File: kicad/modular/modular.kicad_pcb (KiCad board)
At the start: 2 copper layers, 50.5 x 78 mm, 53 parts, among them J1 CONN_PWR, J2 HEADER, J3 HEADER, U1 LM317, U2 LM337, U3 REF5010, U4 OPA4197

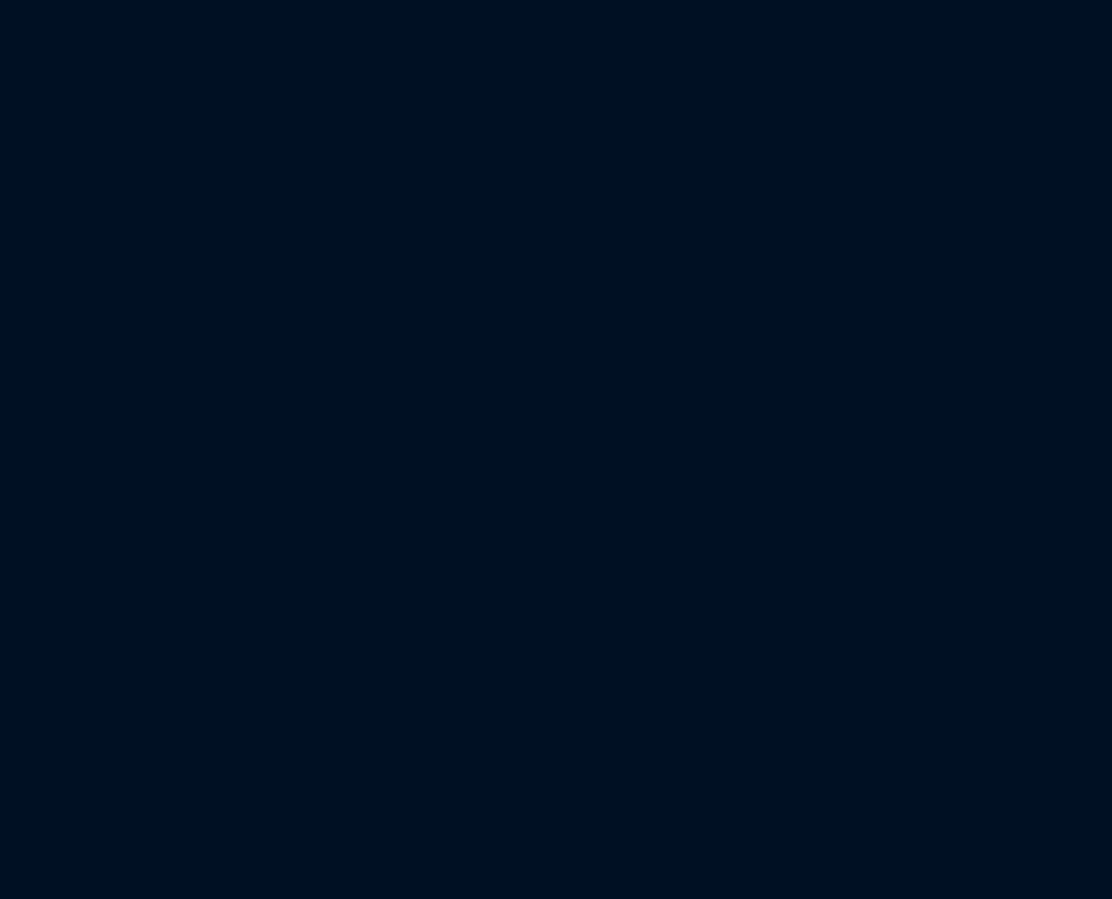
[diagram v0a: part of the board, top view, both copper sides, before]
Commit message: added pcb design of arithmetic board
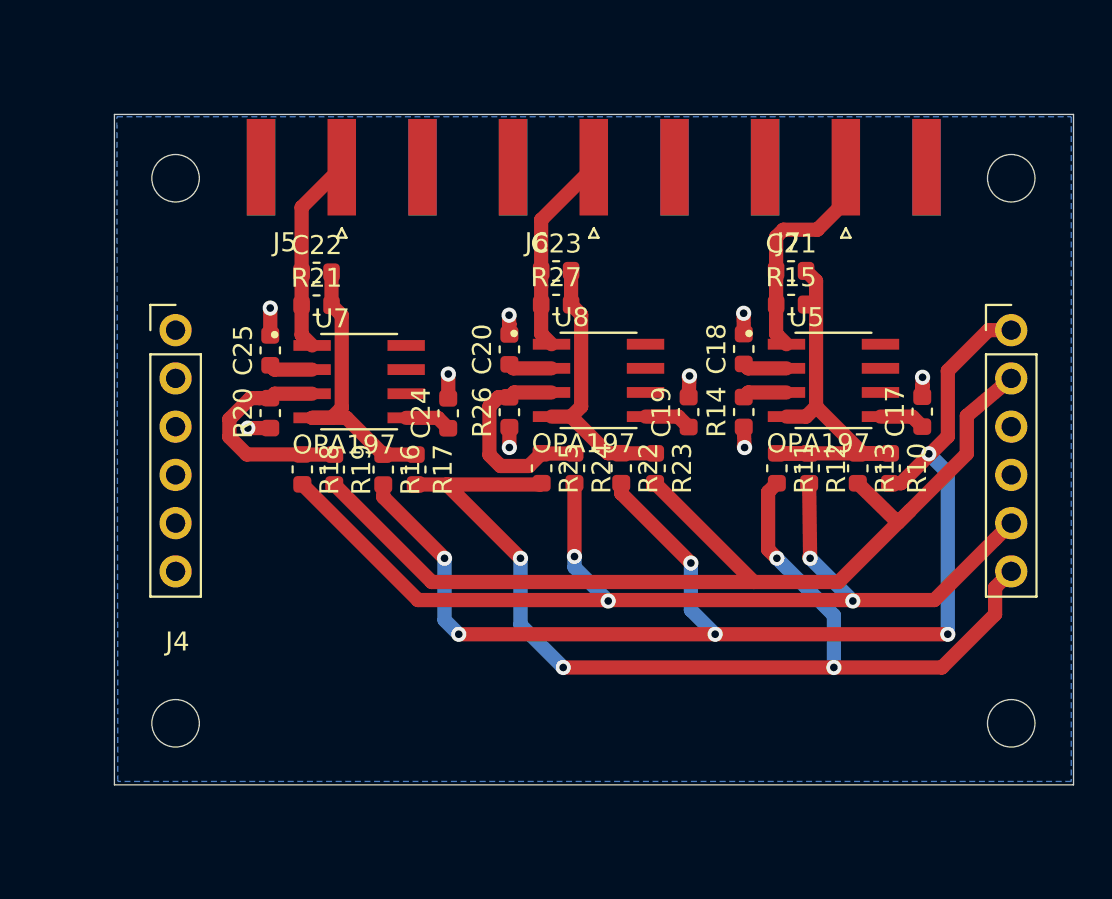
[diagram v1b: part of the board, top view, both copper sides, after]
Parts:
- added C17: 100n, Capacitor_SMD:C_0603_1608Metric, F.Cu at (205.7, 101.8)
- added C18: 100n, Capacitor_SMD:C_0603_1608Metric, F.Cu at (196.3, 98.5)
- added C19: 100n, Capacitor_SMD:C_0603_1608Metric, F.Cu at (193.4, 101.8)
- added C20: 100n, Capacitor_SMD:C_0603_1608Metric, F.Cu at (183.9, 98.5)
- added C21: ?, Capacitor_SMD:C_0603_1608Metric, F.Cu at (198.7, 94.4)
- added C22: ?, Capacitor_SMD:C_0603_1608Metric, F.Cu at (173.8, 94.5)
- added C23: ?, Capacitor_SMD:C_0603_1608Metric, F.Cu at (186.4, 94.4)
- added C24: 100n, Capacitor_SMD:C_0603_1608Metric, F.Cu at (180.7, 101.9)
- added C25: 100n, Capacitor_SMD:C_0603_1608Metric, F.Cu at (171.3, 98.6)
- added J4: Header, Connector_Header:PinHeader_2.54mm, F.Cu at (166.3, 97.5)
- added J5: DIFFX, Connector_Coaxial:SMA_Amphenol_132289_EdgeMount, F.Cu at (175.1, 88.9)
- added J6: DIFFY, Connector_Coaxial:SMA_Amphenol_132289_EdgeMount, F.Cu at (188.4, 88.9)
- added J7: SUM, Connector_Coaxial:SMA_Amphenol_132289_EdgeMount, F.Cu at (201.6, 88.9)
- added R10: 1k, Resistor_SMD:R_0603_1608Metric, F.Cu at (204.0, 104.8)
- added R11: 1k, Resistor_SMD:R_0603_1608Metric, F.Cu at (198.0, 104.8)
- added R12: 1k, Resistor_SMD:R_0603_1608Metric, F.Cu at (199.7, 104.8)
- added R13: 1k, Resistor_SMD:R_0603_1608Metric, F.Cu at (202.3, 104.8)
- added R14: 1k, Resistor_SMD:R_0603_1608Metric, F.Cu at (196.3, 101.8)
- added R15: 1k, Resistor_SMD:R_0603_1608Metric, F.Cu at (198.8, 96.1)
- added R16: 1k, Resistor_SMD:R_0603_1608Metric, F.Cu at (177.3, 104.8)
- added R17: 1k, Resistor_SMD:R_0603_1608Metric, F.Cu at (179.0, 104.8)
- added R18: 1k, Resistor_SMD:R_0603_1608Metric, F.Cu at (173.0, 104.8)
- added R19: 1k, Resistor_SMD:R_0603_1608Metric, F.Cu at (174.7, 104.8)
- added R20: 1k, Resistor_SMD:R_0603_1608Metric, F.Cu at (171.3, 101.9)
- added R21: 1k, Resistor_SMD:R_0603_1608Metric, F.Cu at (173.8, 96.2)
- added R22: 1k, Resistor_SMD:R_0603_1608Metric, F.Cu at (189.8, 104.8)
- added R23: 1k, Resistor_SMD:R_0603_1608Metric, F.Cu at (191.6, 104.8)
- added R24: 1k, Resistor_SMD:R_0603_1608Metric, F.Cu at (187.3, 104.8)
- added R25: 1k, Resistor_SMD:R_0603_1608Metric, F.Cu at (185.6, 104.8)
- added R26: 1k, Resistor_SMD:R_0603_1608Metric, F.Cu at (183.9, 101.8)
- added R27: 1k, Resistor_SMD:R_0603_1608Metric, F.Cu at (186.4, 96.1)
- added U5: OPA197, OPA197IDR:SOIC127P600X175-8N, F.Cu at (201.0, 100.1)
- added U7: OPA197, OPA197IDR:SOIC127P600X175-8N, F.Cu at (176.0, 100.2)
- added U8: OPA197, OPA197IDR:SOIC127P600X175-8N, F.Cu at (188.6, 100.1)
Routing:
- net /Arithmetic/X2: track 0.00 -> 66.9 mm, vias 0 -> 6
- net /Arithmetic/Y1: track 0.00 -> 56.7 mm, vias 0 -> 4
- net /Arithmetic/X1: track 0.00 -> 55.7 mm, vias 0 -> 4
- net /Arithmetic/Y2: track 0.00 -> 54.5 mm
- net Net-(C21-Pad2): track 0.00 -> 21.7 mm
- net Net-(C22-Pad2): track 0.00 -> 15.4 mm
- net Net-(C23-Pad2): track 0.00 -> 14.4 mm
- net /Arithmetic/SUM: track 0.00 -> 12.1 mm
- net Net-(R18-Pad1): track 0.00 -> 11.8 mm
- net Net-(R24-Pad1): track 0.00 -> 11.1 mm
- net /Arithmetic/DIFFY: track 0.00 -> 10.7 mm
- net /Arithmetic/DIFFX: track 0.00 -> 10.5 mm
- net GND: track 251.0 -> 261.4 mm, vias 27 -> 36
- net +12V: track 115.4 -> 122.7 mm
- net -12V: track 107.8 -> 114.7 mm
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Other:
- board size 50.5 x 78 mm -> 119.1 x 78 mm
